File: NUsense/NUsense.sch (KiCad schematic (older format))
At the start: 0 parts

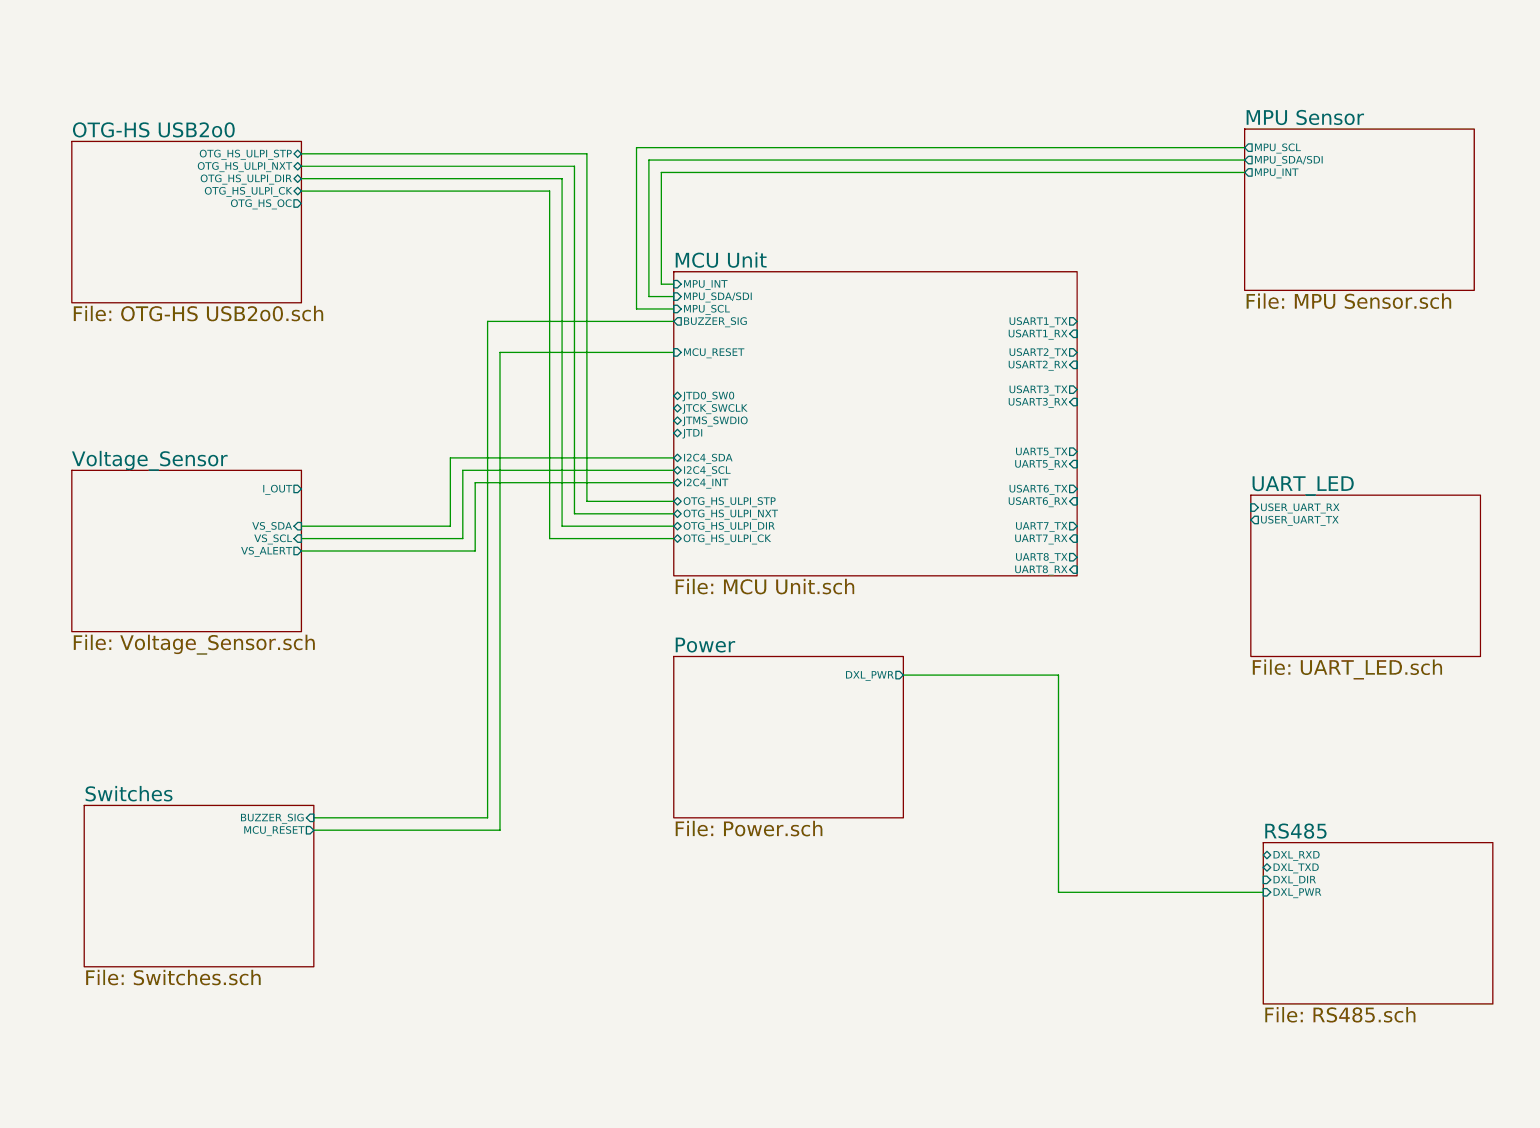
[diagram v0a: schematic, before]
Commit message: Update connections
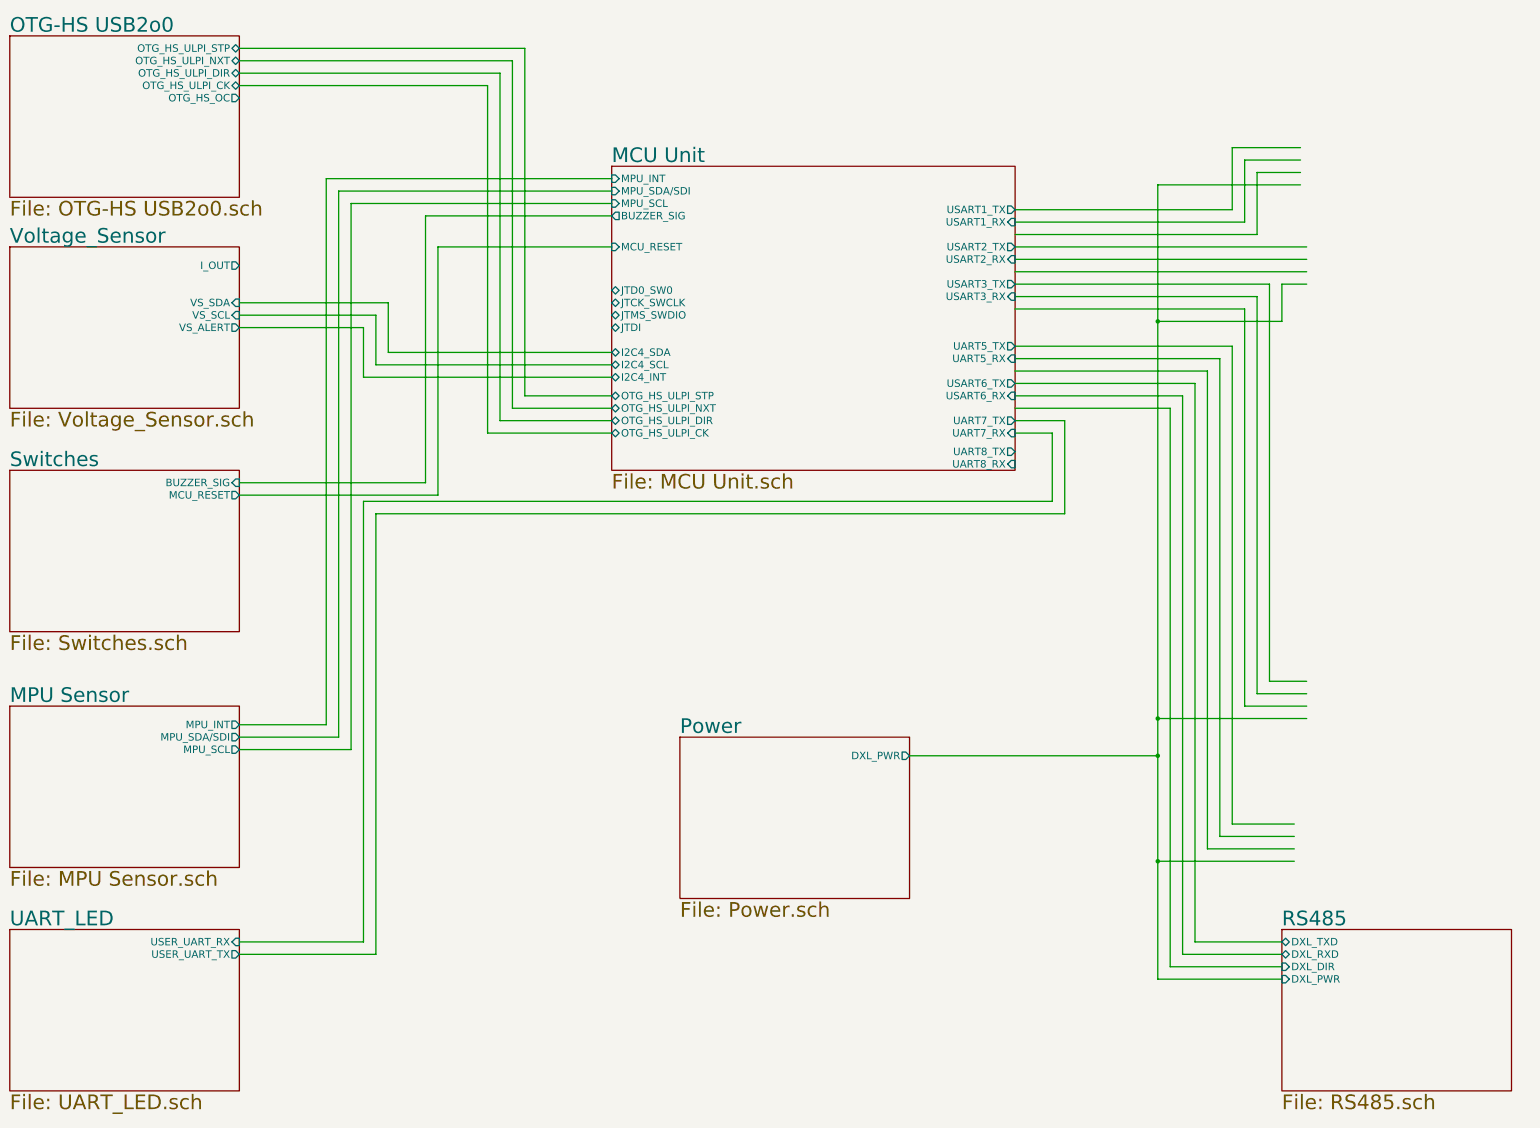
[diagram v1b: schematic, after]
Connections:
- wire segments 39 -> 94
